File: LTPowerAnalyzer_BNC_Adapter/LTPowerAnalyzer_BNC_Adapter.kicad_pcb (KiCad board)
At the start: 2 copper layers, 1 part, among them J1 HTSW-210-08-T-S-RA

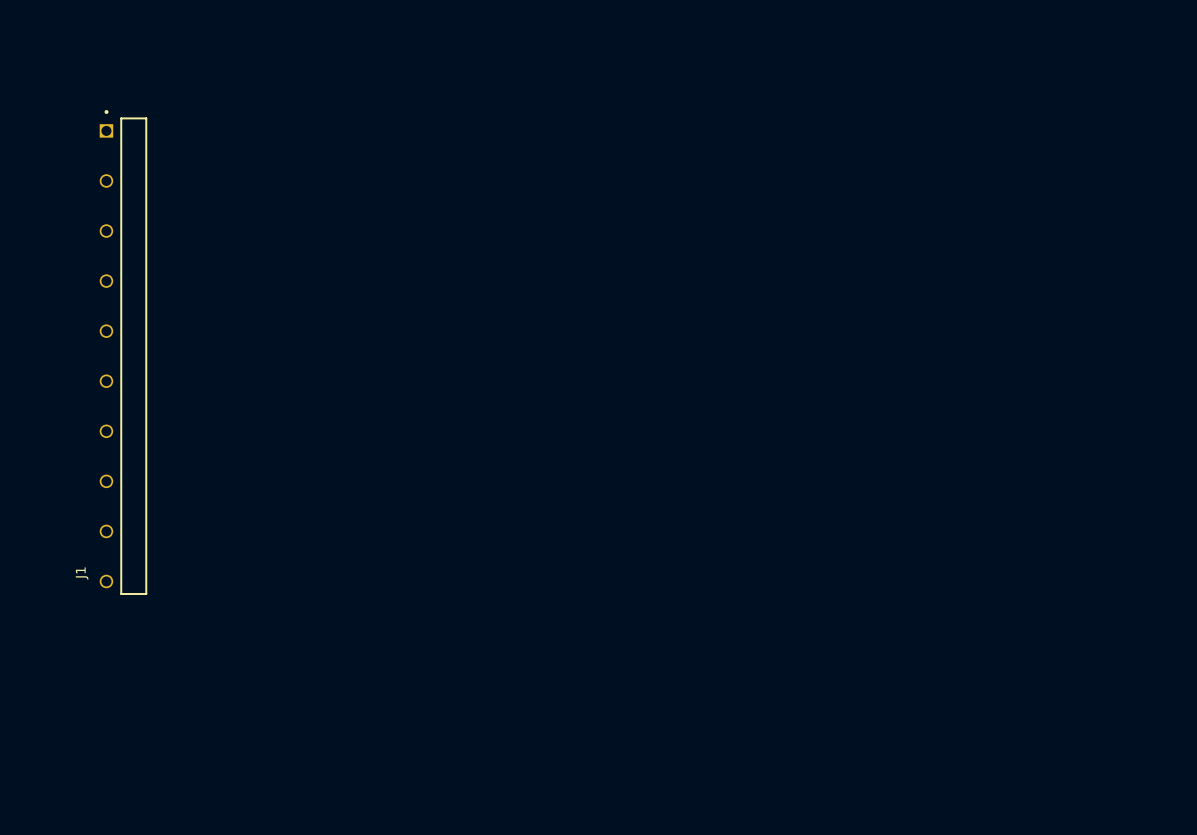
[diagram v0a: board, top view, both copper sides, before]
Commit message: Major update
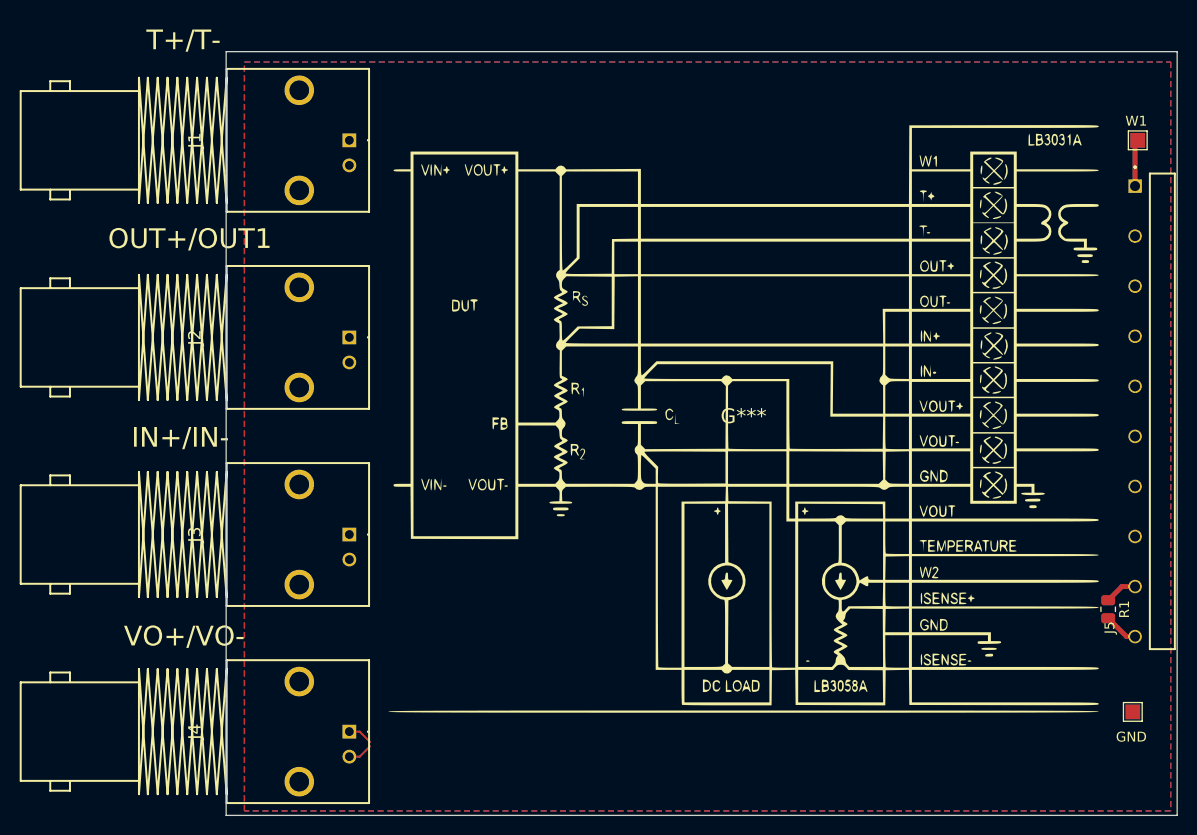
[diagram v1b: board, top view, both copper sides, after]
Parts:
- added G***: LOGO, spencer-connectors:LTPowerAnalyzerConnections, F.Cu at (146.6, 91.0)
- added GND: TestPoint, TestPoint:TestPoint_Pad_1.5x1.5mm, F.Cu at (186.1, 121.0)
- added J1: 031-5431, SamacSys_Parts:0315431, F.Cu at (106.6, 63.0)
- added J2: 031-5431, SamacSys_Parts:0315431, F.Cu at (106.6, 83.0)
- added J3: 031-5431, SamacSys_Parts:0315431, F.Cu at (106.6, 103.0)
- added J4: 031-5431, SamacSys_Parts:0315431, F.Cu at (106.6, 123.0)
- added R1: 0Ω, Resistor_SMD:R_0805_2012Metric, F.Cu at (183.6, 110.5)
- added W1: TestPoint, TestPoint:TestPoint_Pad_1.5x1.5mm, F.Cu at (186.6, 63.0)
- moved J5 104.5 mm to (189.1, 90.5)
- renumbered J1 to J5
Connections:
- J5 pad 01: unconnected-(J1-Pad01) -> /W1
- J5 pad 02: unconnected-(J1-Pad02) -> /T+
- J5 pad 03: unconnected-(J1-Pad03) -> /T-
- J5 pad 04: unconnected-(J1-Pad04) -> /OUT+
- J5 pad 05: unconnected-(J1-Pad05) -> /OUT-
- J5 pad 06: unconnected-(J1-Pad06) -> /IN+
- J5 pad 07: unconnected-(J1-Pad07) -> /IN-
- J5 pad 08: unconnected-(J1-Pad08) -> /VO+
- J5 pad 09: unconnected-(J1-Pad09) -> /VO-
- J5 pad 10: unconnected-(J1-Pad10) -> GND
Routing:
- net /VO-: track 0.00 -> 92.1 mm
- net /VO+: track 0.00 -> 88.8 mm
- net /T-: track 0.00 -> 85.7 mm
- net /IN+: track 0.00 -> 84.7 mm
- net /IN-: track 0.00 -> 84.7 mm
- net /T+: track 0.00 -> 83.8 mm
- net /OUT-: track 0.00 -> 81.6 mm
- net /OUT+: track 0.00 -> 81.6 mm
- net /W1: track 0.00 -> 4.75 mm
- net GND: track 0.00 -> 3.50 mm
- added copper zone on B.Cu, net GND
- added copper zone on F.Cu, net GND
- added copper zone on In1.Cu, net GND
- added copper zone on In2.Cu, net GND
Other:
- board outline added: 96.5 x 77.5 mm
- copper layers 2 -> 4
- board text added: "IN+/IN-"
- board text added: "OUT+/OUT1"
- board text added: "T+/T-"
- board text added: "VO+/VO-"
